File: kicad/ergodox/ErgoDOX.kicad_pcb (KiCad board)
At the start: 2 copper layers, 182.8 x 158.9 mm, 65 parts, among them J1 USB, J2 3.5mm, J3 JMP, J4 JMP, SW0:10 SW0:3, SW0:11 SW0:2, SW0:12 SW0:1, SW0:7 SW0:6, SW0:8 SW0:5, SW0:9 SW0:4, SW1:10 SW1:3, SW1:11 SW1:2, SW1:12 SW1:1, SW1:13 SW1:0, SW1:9 SW1:4, SW2:10 SW2:3, SW2:11 SW2:2, SW2:12 SW2:1, SW2:13 SW2:0, SW2:7 SW2:6, SW2:8 SW2:5, SW2:9 SW2:4, SW3:10 SW3:3, SW3:11 SW3:2, SW3:12 SW3:1, SW3:13 SW3:0, SW3:8 SW3:5, SW3:9 SW3:4, SW4:10 SW4:3, SW4:11 SW4:2, SW4:12 SW4:1, SW4:13 SW4:0, SW4:7 SW4:6, SW4:8 SW4:5, SW4:9 SW4:4, SW5:10 SW5:3, SW5:11 SW5:2, SW5:12 SW5:1, SW5:13 SW5:0, SW5:7 SW5:6, SW5:8 SW5:5, SW5:9 SW5:4, U1 TEENSY2.0, U2 MCP23018

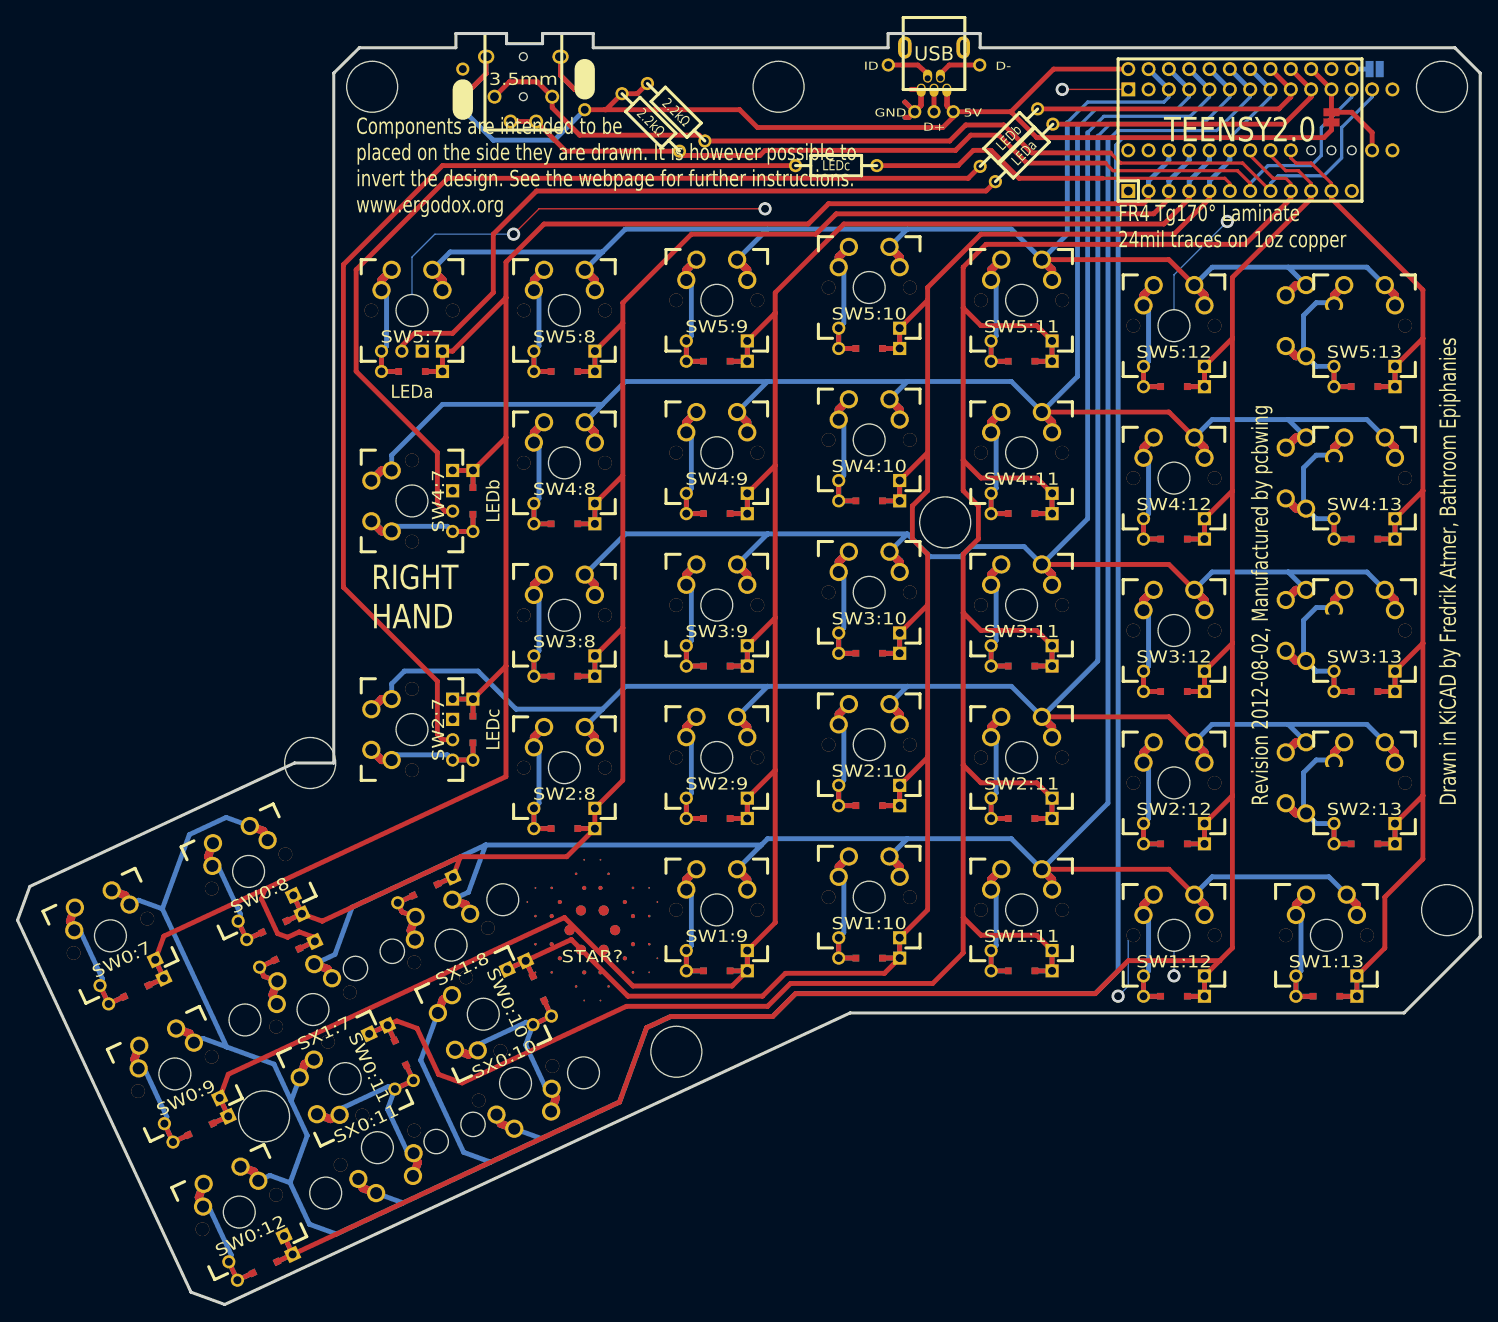
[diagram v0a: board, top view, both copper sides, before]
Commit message: update ergodox kicad project kicad 5
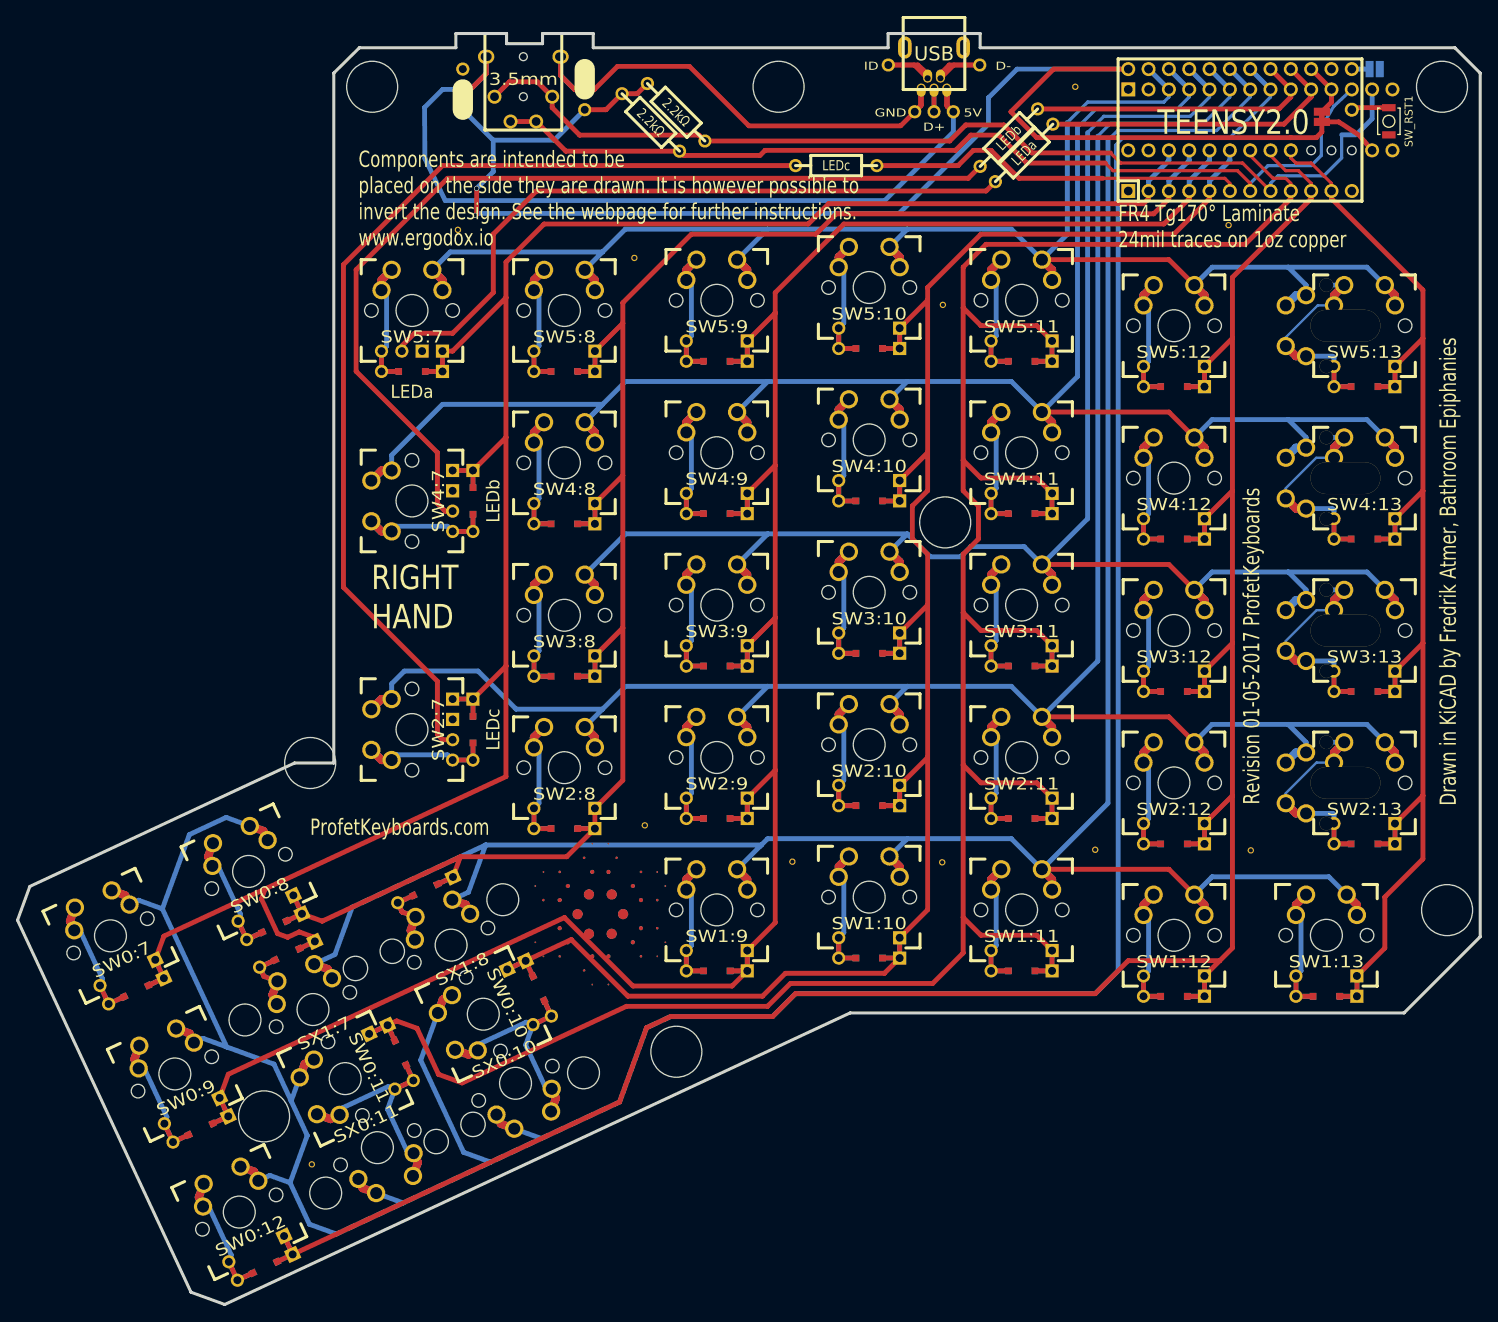
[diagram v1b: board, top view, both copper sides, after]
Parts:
- removed STAR? (x2): STAR, STAR
- added STAR_1: STAR_FRONT, ErgoDOX pcb:STAR, F.Cu at (95.9, 140.6)
- added STAR_2: STAR_BACK, ErgoDOX pcb:STAR, B.Cu at (95.9, 140.6)
- added STITCHING_VIA: ~, lib_footprints:STITCHING_VIA, F.Cu at (100.2, 58.5)
- added STITCHING_VIA: ~, lib_footprints:STITCHING_VIA, F.Cu at (78.1, 55.0)
- added STITCHING_VIA: ~, lib_footprints:STITCHING_VIA, F.Cu at (138.8, 64.4)
- added STITCHING_VIA: ~, lib_footprints:STITCHING_VIA, F.Cu at (177.2, 132.6)
- added STITCHING_VIA: ~, lib_footprints:STITCHING_VIA, F.Cu at (157.8, 132.5)
- added STITCHING_VIA: ~, lib_footprints:STITCHING_VIA, F.Cu at (138.7, 134.1)
- added STITCHING_VIA: ~, lib_footprints:STITCHING_VIA, F.Cu at (119.9, 134.0)
- added STITCHING_VIA: ~, lib_footprints:STITCHING_VIA, F.Cu at (59.9, 171.8)
- added STITCHING_VIA: ~, lib_footprints:STITCHING_VIA, F.Cu at (101.5, 129.5)
- added STITCHING_VIA: ~, lib_footprints:STITCHING_VIA, F.Cu at (155.3, 37.1)
- added STITCHING_VIA: ~, lib_footprints:STITCHING_VIA, F.Cu at (174.5, 54.4)
- added SW_RST1: SWITCH_PUSH, Buttons_Switches_SMD:SW_SPST_B3U-1000P, F.Cu at (194.5, 41.5)
- SW0:10, SW0:11, SW0:12, SW0:7, SW0:8, SW0:9, SW1:10, SW1:11, SW1:12, SW1:13, SW1:9, SW2:10, SW2:11, SW2:12, SW2:7, SW2:8, SW2:9, SW3:10, SW3:11, SW3:12, SW3:8, SW3:9, SW4:10, SW4:11, SW4:12, SW4:7, SW4:8, SW4:9, SW5:10, SW5:11, SW5:12, SW5:7, SW5:8, SW5:9: footprint MX_FLIP_DIODE -> ErgoDOX pcb:MX_FLIP_DIODE
- SW2:13, SW3:13, SW4:13, SW5:13: footprint MX_FLIP_XX -> ErgoDOX pcb:MX_FLIP_XX
- U1: footprint TEENSY_2.0 -> ErgoDOX pcb:TEENSY_2.0_WITH_RESET
- moved SW2:13 4.76 mm to (191.5, 124.2)
- moved SW3:13 4.76 mm to (191.5, 105.1)
- moved SW4:13 4.76 mm to (191.5, 86.1)
- moved SW5:13 4.76 mm to (191.5, 67.0)
- moved JP1 1.20 mm to (186.1, 40.9)
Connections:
- J1 pad 1: VCC -> Net-(J1-Pad1)
- J1 pad 2: (no net) -> Net-(J1-Pad2)
- J1 pad 3: (no net) -> Net-(J1-Pad3)
- J1 pad 4: (no net) -> Net-(J1-Pad4)
- J1 pad 5: GND -> Net-(J1-Pad5)
- J2 pad 1: N-000003 -> Net-(J1-Pad5)
- J2 pad 4: N-000001 -> Net-(J1-Pad1)
- J3 pad 2: N-000003 -> Net-(J1-Pad5)
- J4 pad 2: N-000001 -> Net-(J1-Pad1)
- U1 pad 12: (no net) -> Net-(U1-Pad12)
- U1 pad 19: (no net) -> Net-(U1-Pad19)
- U2 pad 10: (no net) -> /LED_A
- U2 pad 14: (no net) -> Net-(U2-Pad14)
- U2 pad 17: (no net) -> Net-(U2-Pad17)
- U2 pad 18: (no net) -> Net-(U2-Pad18)
- U2 pad 19: (no net) -> Net-(U2-Pad19)
- U2 pad 27: (no net) -> Net-(U2-Pad27)
- U2 pad 28: (no net) -> Net-(U2-Pad28)
- U2 pad 9: (no net) -> /LED_B
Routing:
- net Net-(J1-Pad1): track 0.00 -> 102.6 mm
- net GND: track 104.3 -> 2.22 mm, vias 6 -> 0
- net Net-(J1-Pad5): track 0.00 -> 62.3 mm
- net VCC: track 160.4 -> 204.8 mm, vias 0 -> 2
- net N-000003: track 12.2 -> 0.00 mm
- net N-000001: track 11.7 -> 0.00 mm
- net Net-(SW3:13-Pad2): track 31.2 -> 38.1 mm
- net Net-(SW4:13-Pad2): track 31.2 -> 38.1 mm
- net Net-(SW5:13-Pad2): track 31.2 -> 38.0 mm
- net Net-(SW2:13-Pad2): track 31.2 -> 37.7 mm
- net Net-(J1-Pad4): track 0.00 -> 5.60 mm
- net Net-(J1-Pad2): track 0.00 -> 5.60 mm
- net /RST: track 0.00 -> 4.74 mm
- net Net-(J1-Pad3): track 0.00 -> 2.98 mm
- net /ROW4: track 259.2 -> 257.4 mm
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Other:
- net class Default: trace_width 0.3048 -> 0.6
- board text added: "Components are intended to be placed on the side they are drawn. It is however possible to invert the design. See the webpage for further instructions. www.ergodox.io"
- board text added: "ProfetKeyboards.com"
- board text added: "Revision 01-05-2017 ProfetKeyboards"
- board text removed: "Components are intended to be placed on the side they are drawn. It is however possible to invert the design. See the webpage for further instructions. www.ergodox.org"
- board text removed: "Revision 2012-08-02, Manufactured by pcbwing"
